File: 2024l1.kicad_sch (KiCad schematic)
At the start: 0 parts

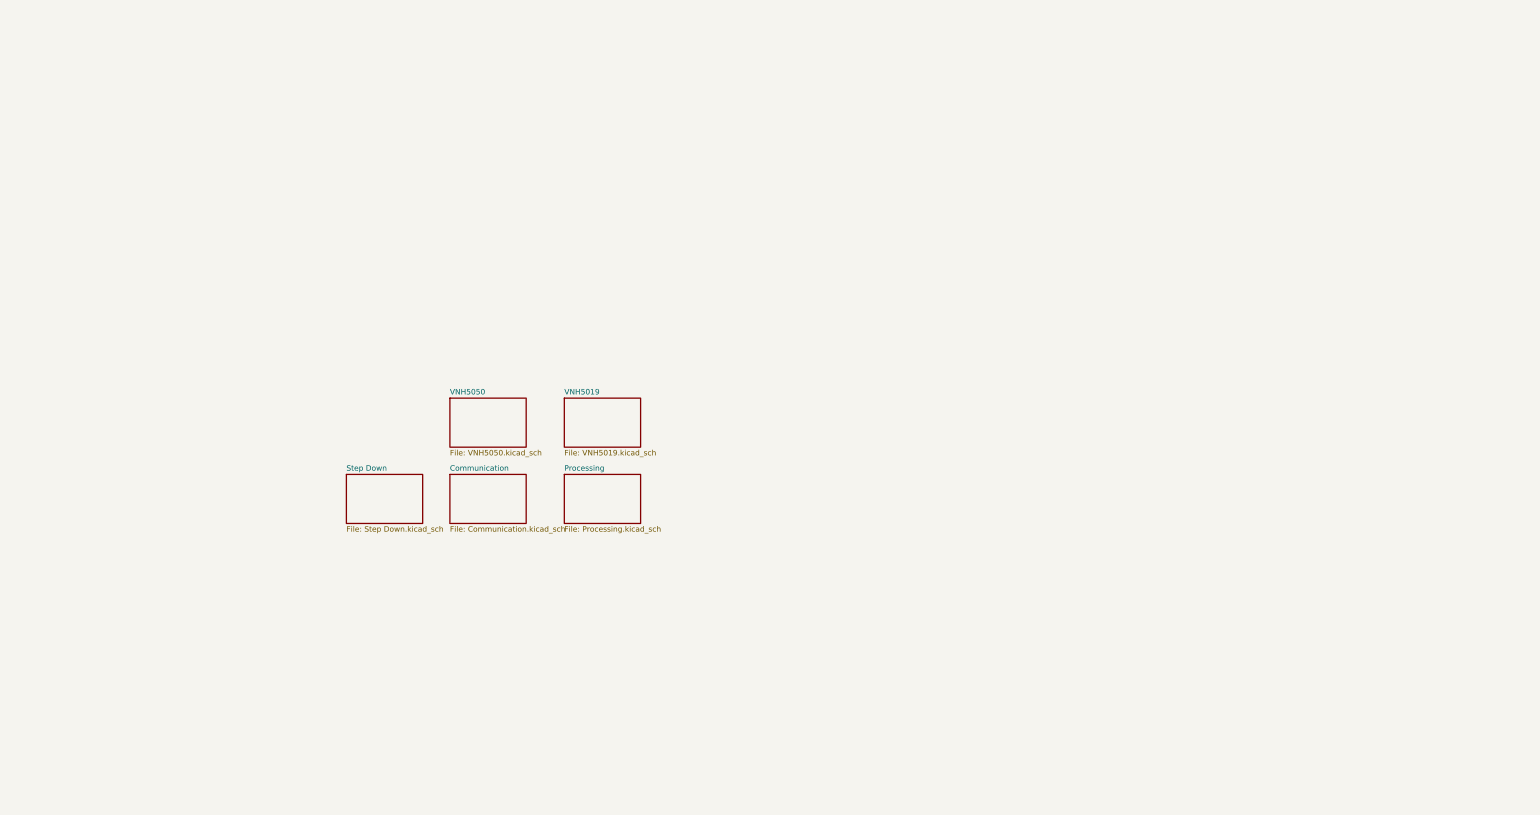
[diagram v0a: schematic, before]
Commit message: Rethought L1
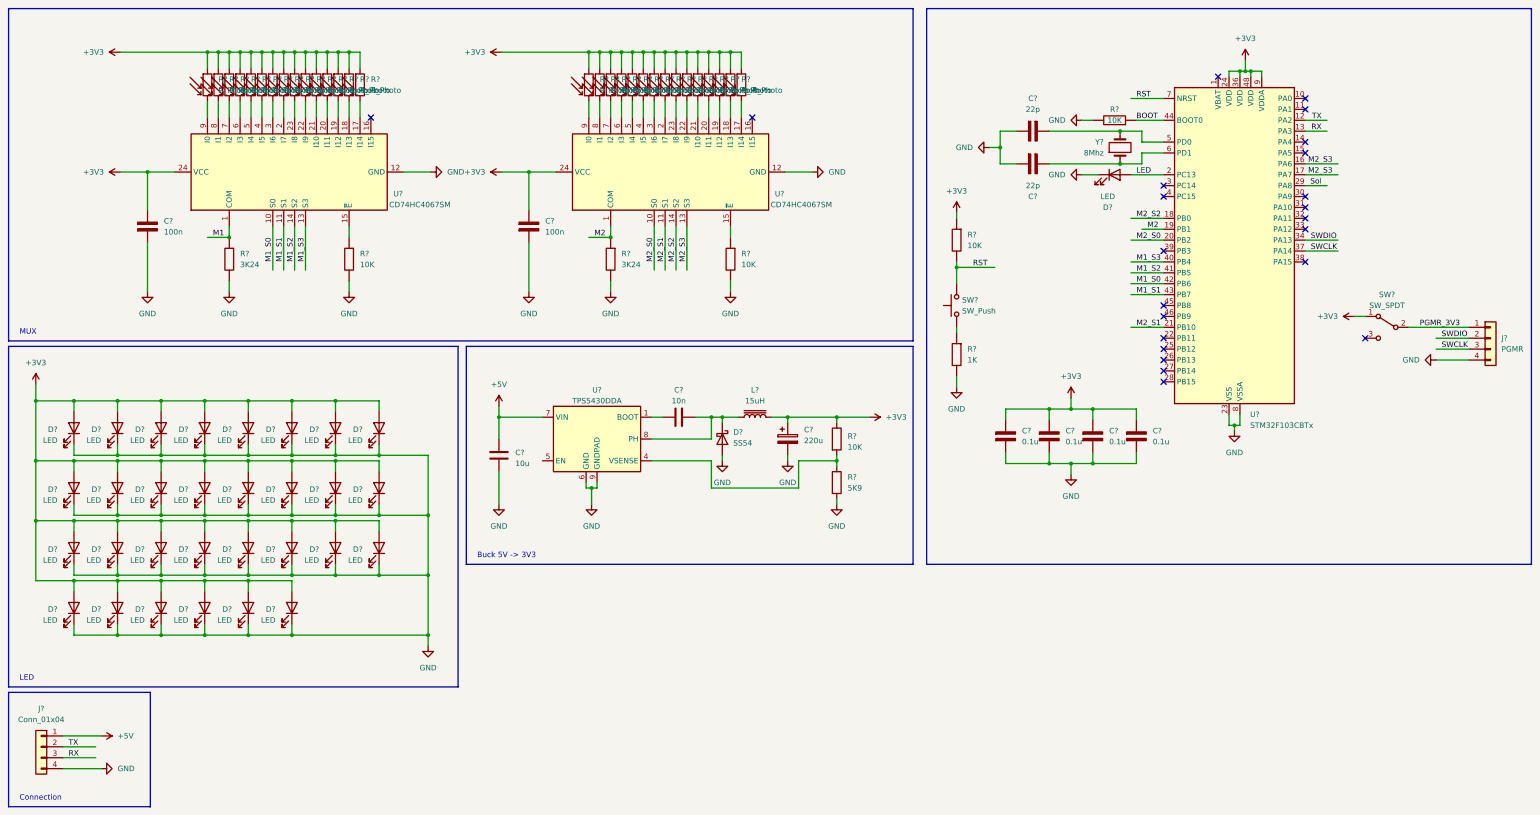
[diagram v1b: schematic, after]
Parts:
- added C? (x4): 0.1u, symbol vincent:C
- added C? (x2): 100n, symbol vincent:C
- added C? (x2): 22p, symbol vincent:C
- added C?: 10n, footprints:cap0603, symbol Device:C
- added C?: 10u, footprints:cap0603, symbol Device:C
- added C?: 220u, footprints:EIA-7343-D, symbol Device:C_Polarized
- added D? (x31): LED, symbol Device:LED
- added D?: SS54, footprints:DIOM5025X220N, symbol Diode:B340
- added J?: Conn_01x04, symbol Connector_Generic:Conn_01x04
- added J?: PGMR, symbol Connector_Generic:Conn_01x04
- added L?: 15uH, footprints:0630 One Piece Inductor, symbol Device:L_Iron
- added R? (x30): R_Photo, symbol Device:R_Photo
- added R? (x4): 10K, symbol vincent:R
- added R?: 1K, symbol vincent:R
- added R?: 5K9, footprints:res0603, symbol Device:R
- added R? (x2): 3K24, symbol vincent:R
- added R?: 10K, footprints:res0603, symbol Device:R
- added SW?: SW_Push, symbol Switch:SW_Push
- added SW?: SW_SPDT, symbol Switch:SW_SPDT
- added U?: TPS5430DDA, footprints:TI_SO-PowerPAD-8_ThermalVias, symbol Regulator_Switching:TPS5430DDA
- added U?: STM32F103CBTx, Package_QFP:LQFP-48_7x7mm_P0.5mm, symbol vincent:STM32F103CBTx
- added U? (x2): CD74HC4067SM, Package_SO:SSOP-24_5.3x8.2mm_P0.65mm, symbol 74xx:CD74HC4067SM
- added Y?: 8Mhz, symbol vincent:Crystal
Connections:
- new net: R?.2, U?.9 (I0) (x2)
- new net: R?.2, U?.17 (I14) (x2)
- new net: R?.2, U?.15 (~{E}) (x2)
- new net: R?.2, U?.2 (I7) (x2)
- new net: R?.2, SW?.1
- new net: C?.2, D?.1 (K), L?.1, U?.8 (PH)
- new net: R?.2, U?.8 (I1) (x2)
- new net: R?.2, U?.5 (I4) (x2)
- new net: R?.2, U?.4 (I5) (x2)
- new net: R?.2, U?.22 (I9) (x2)
- new net: R?.2, U?.19 (I12) (x2)
- new net: C?.2, U?.5 (PD0), Y?.2
- new net: R?.2, U?.7 (I2) (x2)
- new net: R?.2, U?.3 (I6) (x2)
- new net: R?.2, U?.18 (I13) (x2)
- new net: R?.1, R?.2, U?.4 (VSENSE)
- new net: C?.2, U?.6 (PD1), Y?.1
- new net: R?.2, U?.23 (I8) (x2)
- new net: C?.1, U?.1 (BOOT)
- new net: R?.2, U?.20 (I11) (x2)
- new net: R?.2, U?.6 (I3) (x2)
- new net: R?.2, U?.21 (I10) (x2)
- new net +3V3: C?.1, C?.2, C?.2, C?.2, C?.2, C?.2, C?.2, D?.2 (A), D?.2 (A), D?.2 (A), D?.2 (A), D?.2 (A), D?.2 (A), D?.2 (A), D?.2 (A), D?.2 (A), D?.2 (A), D?.2 (A), D?.2 (A), D?.2 (A), D?.2 (A), D?.2 (A), D?.2 (A), D?.2 (A), D?.2 (A), D?.2 (A), D?.2 (A), D?.2 (A), D?.2 (A), D?.2 (A), D?.2 (A), D?.2 (A), D?.2 (A), D?.2 (A), D?.2 (A), D?.2 (A), D?.2 (A), L?.2, R?.1, R?.1, R?.1, R?.1, R?.1, R?.1, R?.1, R?.1, R?.1, R?.1, R?.1, R?.1, R?.1, R?.1, R?.1, R?.1, R?.1, R?.1, R?.1, R?.1, R?.1, R?.1, R?.1, R?.1, R?.1, R?.1, R?.1, R?.1, R?.1, R?.1, R?.1, R?.2, SW?.1 (A), U?.24 (VCC), U?.24 (VCC), U?.24 (VDD), U?.36 (VDD), U?.48 (VDD), U?.9 (VDDA)
- new net +5V: C?.1, J?.1 (Pin_1), U?.7 (VIN)
- new net BOOT: R?.2, U?.44 (BOOT0)
- new net GND: C?.1, C?.1, C?.1, C?.1, C?.1, C?.1, C?.1, C?.1, C?.2, C?.2, D?.1 (K), D?.1 (K), D?.1 (K), D?.1 (K), D?.1 (K), D?.1 (K), D?.1 (K), D?.1 (K), D?.1 (K), D?.1 (K), D?.1 (K), D?.1 (K), D?.1 (K), D?.1 (K), D?.1 (K), D?.1 (K), D?.1 (K), D?.1 (K), D?.1 (K), D?.1 (K), D?.1 (K), D?.1 (K), D?.1 (K), D?.1 (K), D?.1 (K), D?.1 (K), D?.1 (K), D?.1 (K), D?.1 (K), D?.1 (K), D?.1 (K), D?.2 (A), J?.4 (Pin_4), J?.4 (Pin_4), R?.1, R?.1, R?.1, R?.1, R?.1, R?.1, R?.2, U?.12 (GND), U?.12 (GND), U?.23 (VSS), U?.35 (VSS), U?.47 (VSS), U?.6 (GND), U?.8 (VSSA), U?.9 (GNDPAD)
- new net LED: D?.2 (A), U?.2 (PC13)
- new net M1: R?.2, U?.1 (COM)
- new net M1_S0: U?.10 (S0), U?.42 (PB6)
- new net M1_S1: U?.11 (S1), U?.43 (PB7)
- new net M1_S2: U?.14 (S2), U?.41 (PB5)
- new net M1_S3: U?.13 (S3), U?.40 (PB4)
- new net M2: R?.2, U?.1 (COM), U?.19 (PB1)
- new net M2_S0: U?.10 (S0), U?.20 (PB2)
- new net M2_S1: U?.11 (S1), U?.21 (PB10)
- new net M2_S2: U?.14 (S2), U?.18 (PB0)
- new net M2_S3: U?.13 (S3), U?.16 (PA6), U?.17 (PA7)
- new net PGMR_3V3: J?.1 (Pin_1), SW?.2 (B)
- new net RST: R?.1, SW?.2, U?.7 (NRST)
- new net RX: J?.3 (Pin_3), U?.13 (PA3)
- new net SWCLK: J?.3 (Pin_3), U?.37 (PA14)
- new net SWDIO: J?.2 (Pin_2), U?.34 (PA13)
- new net Sol: U?.29 (PA8)
- new net TX: J?.2 (Pin_2), U?.12 (PA2)
- no-connect marks 0 -> 23
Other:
- removed sheet Communication
- removed sheet Processing
- removed sheet Step Down
- removed sheet VNH5019
- removed sheet VNH5050
- note added: "Buck 5V -> 3V3"
- note added: "Connection"
- note added: "LED"
- note added: "MUX"
